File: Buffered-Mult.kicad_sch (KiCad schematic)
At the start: 53 parts, among them J1 Eurorack PWR, J10 OUTPUT2-3, J11 OUTPUT3-1, J12 OUTPUT3-2, J13 OUTPUT3-3, J2 INPUT1, J3 INPUT2, J4 INPUT3, J5 OUTPUT1-1, J6 OUTPUT1-2, J7 OUTPUT1-3, J8 OUTPUT2-1, J9 OUTPUT2-2, U1 TL074, U2 TL074, U3 TL074

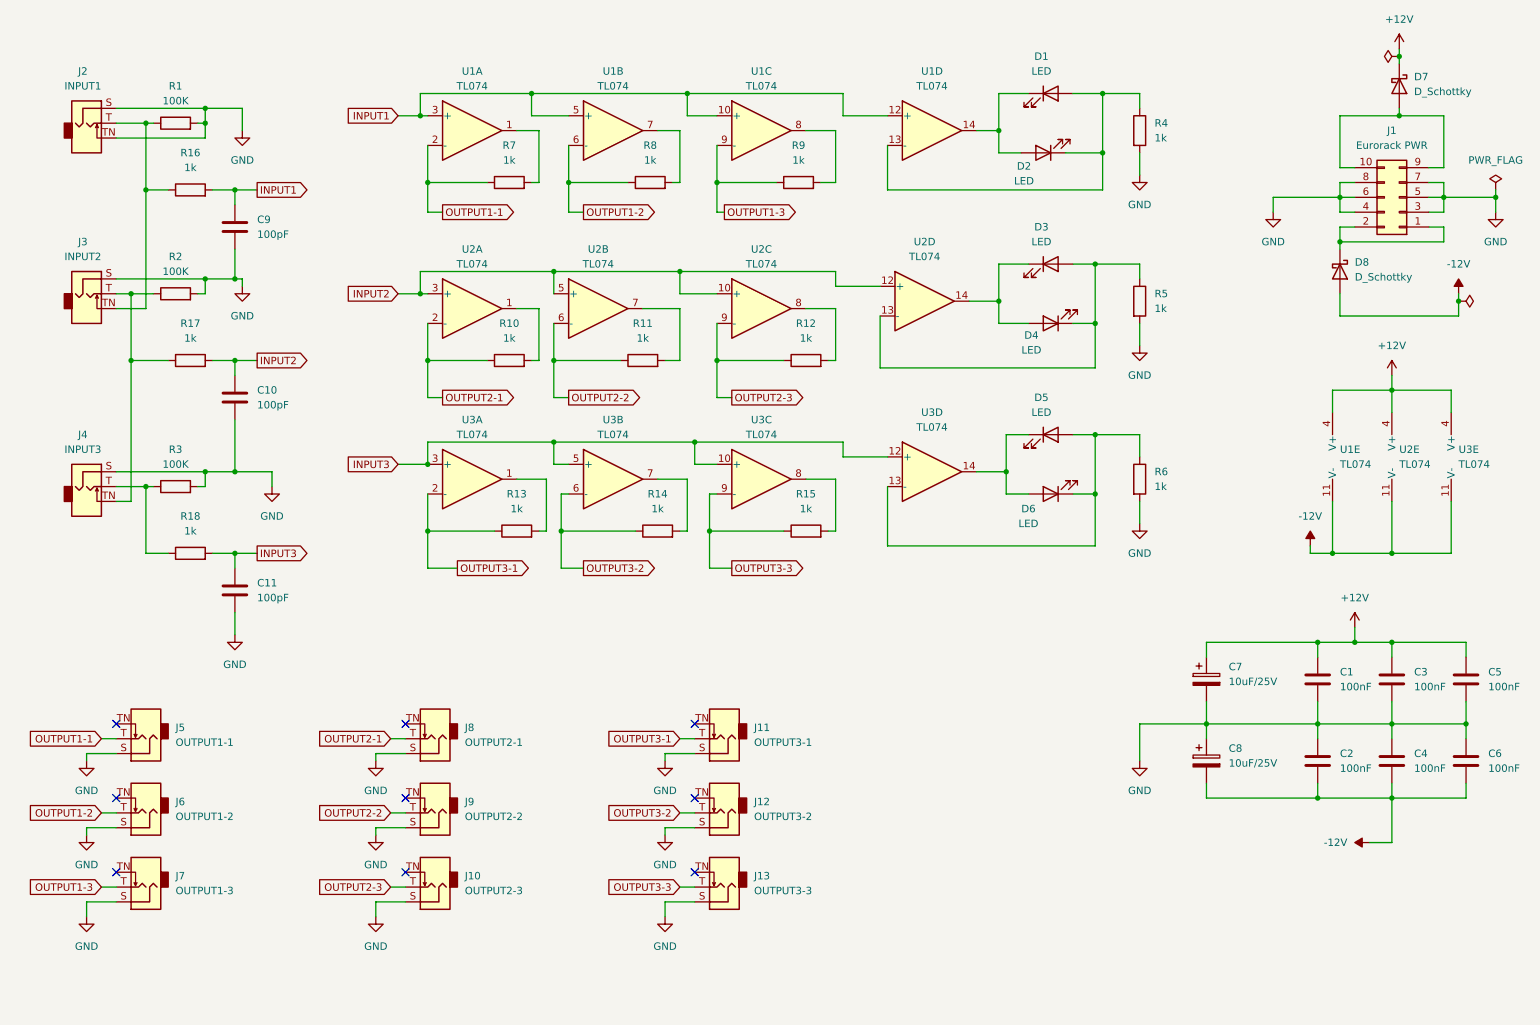
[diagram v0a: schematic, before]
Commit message: Updated schematic
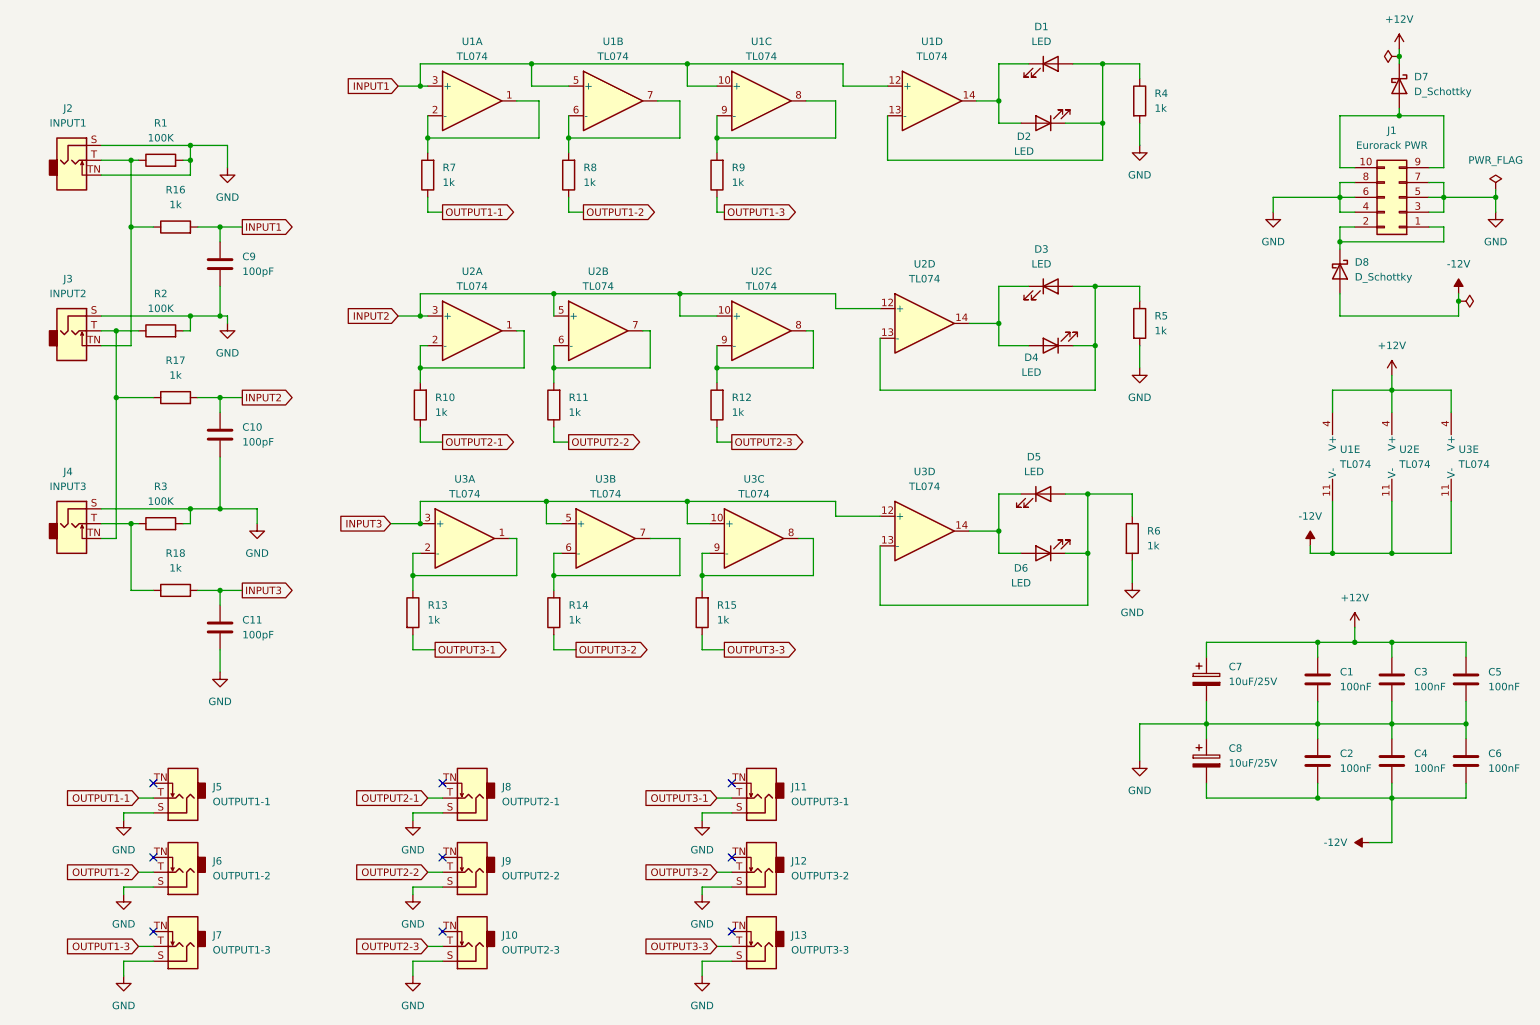
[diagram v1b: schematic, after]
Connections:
- net OUTPUT1-1: no longer U1.2 (-)
- net OUTPUT1-2: no longer U1.6 (-)
- net OUTPUT1-3: no longer U1.9 (-)
- net OUTPUT2-1: no longer U2.2 (-)
- net OUTPUT2-2: no longer U2.6 (-)
- net OUTPUT2-3: no longer U2.9 (-)
- net OUTPUT3-1: now also R13.2; no longer R13.1, U3.2 (-)
- net OUTPUT3-2: no longer U3.6 (-)
- net OUTPUT3-3: no longer U3.9 (-)
- net at R8.2, U1.7: now also U1.6 (-)
- net at R12.2, U2.8: now also U2.9 (-)
- net at R11.2, U2.7: now also U2.6 (-)
- net at R7.2, U1.1: now also U1.2 (-)
- net at R10.2, U2.1: now also U2.2 (-)
- net at R15.2, U3.8: now also U3.9 (-)
- net at R9.2, U1.8: now also U1.9 (-)
- net at U3.1: now also R13.1, U3.2 (-); no longer R13.2
- net at R14.2, U3.7: now also U3.6 (-)
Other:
- moved on the sheet: C10, C11, C9, D1, D2, D3, D4, D5, D6, J10, J11, J12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

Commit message: Add LCSC Part numbers
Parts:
- C1, C2, C3, C4, C5, C6: footprint (none) -> Capacitor_SMD:C_0603_1608Metric_Pad1.08x0.95mm_HandSolder; LCSC (none) -> C14663
- C10, C11, C9: footprint (none) -> Capacitor_SMD:C_0603_1608Metric_Pad1.08x0.95mm_HandSolder; LCSC (none) -> C14858
- C7, C8: footprint (none) -> Capacitor_SMD:CP_Elec_5x3; LCSC (none) -> C46550416
- D1, D2, D3, D4, D5, D6: footprint (none) -> LED_THT:LED_D3.0mm_FlatTop
- D7, D8: footprint (none) -> Diode_SMD:D_SOD-323; LCSC (none) -> C2480
- J1: footprint (none) -> Connector_IDC:IDC-Header_2x05_P2.54mm_Vertical
- J10, J11, J12, J13, J2, J3, J4, J5, J6, J7, J8, J9: footprint (none) -> Connector_Audio:Jack_3.5mm_QingPu_WQP-PJ398SM_Vertical_CircularHoles
- R1, R2, R3: footprint (none) -> Resistor_SMD:R_0603_1608Metric_Pad0.98x0.95mm_HandSolder; LCSC (none) -> C25803
- R10, R11, R12, R13, R14, R15, R16, R17, R18, R4, R5, R6, R7, R8, R9: footprint (none) -> Resistor_SMD:R_0603_1608Metric_Pad0.98x0.95mm_HandSolder; LCSC (none) -> C21190
- U1, U2, U3: footprint (none) -> Package_SO:SOIC-14_3.9x8.7mm_P1.27mm; LCSC (none) -> C2878713

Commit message: First draft of PCB
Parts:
- C7, C8: footprint Capacitor_SMD:CP_Elec_5x3 -> Capacitor_SMD:CP_Elec_5x5.4
- D7, D8: footprint Diode_SMD:D_SOD-323 -> Diode_SMD:D_SMA_Handsoldering
